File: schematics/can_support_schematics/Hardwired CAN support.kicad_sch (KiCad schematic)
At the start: 27 parts, among them J1 Programming Connector, J2 Conn_01x05_Male, J3 Conn_01x05_Male, J4 Screw_Terminal_01x02, J5 Screw_Terminal_01x04, SW1 SW_DIP_x04, U1 PIC18F26K83, U2 TCAN1042VDQ1, Y1 Crystal

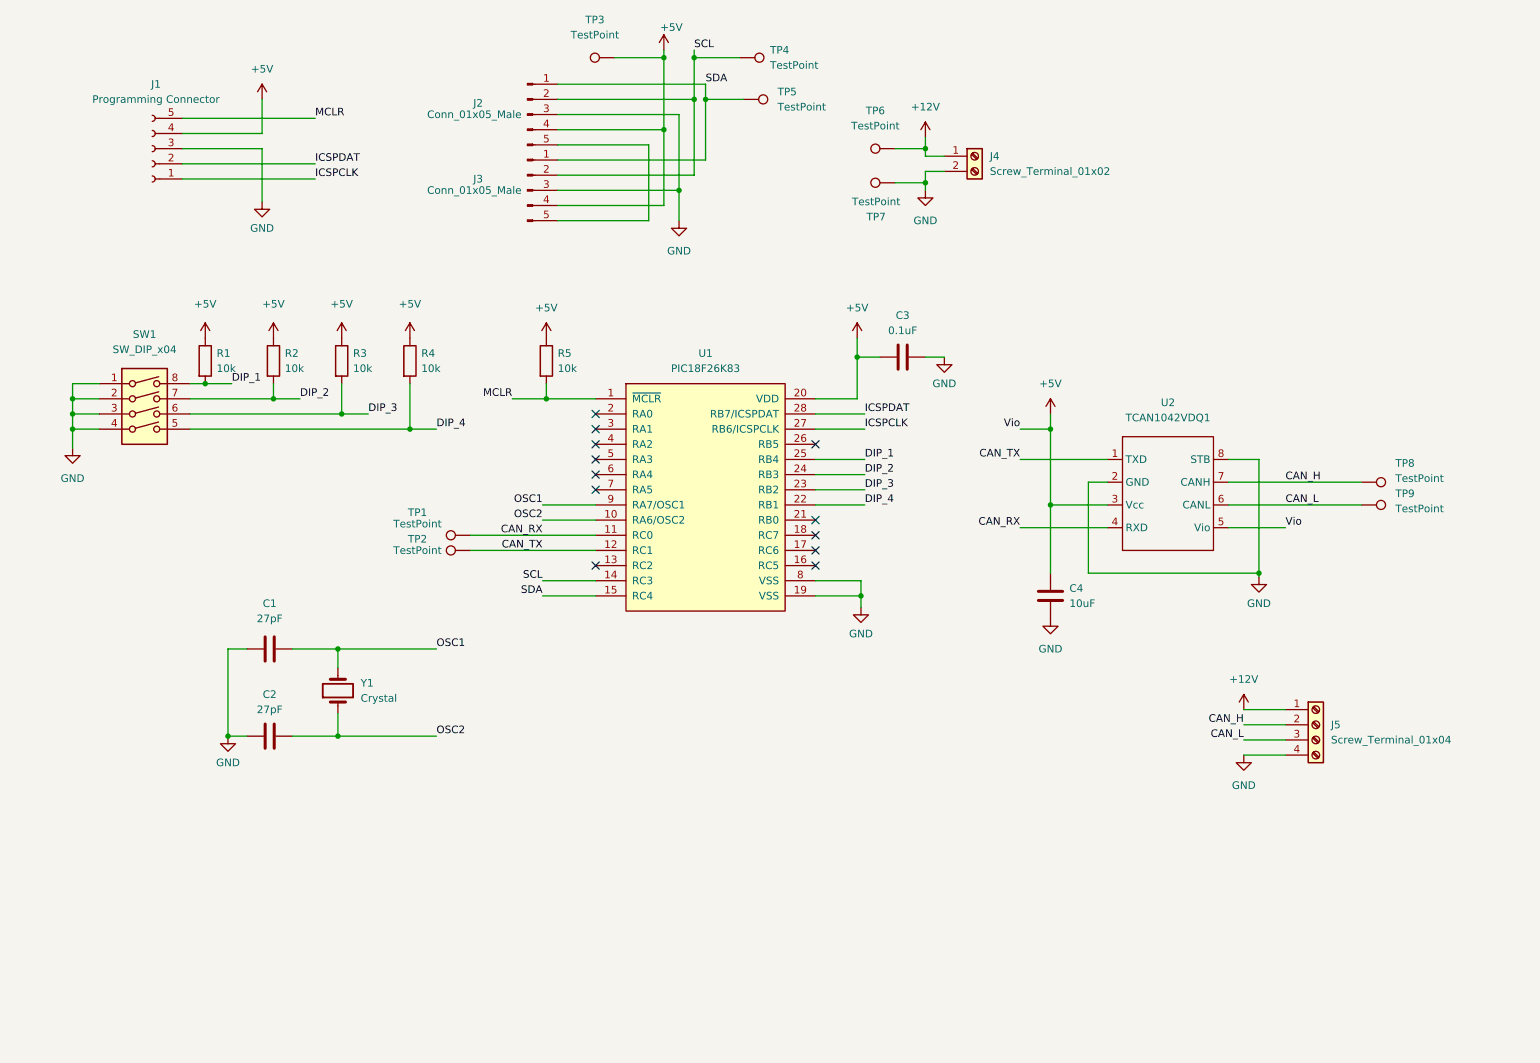
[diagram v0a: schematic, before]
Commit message: Stuff Updated
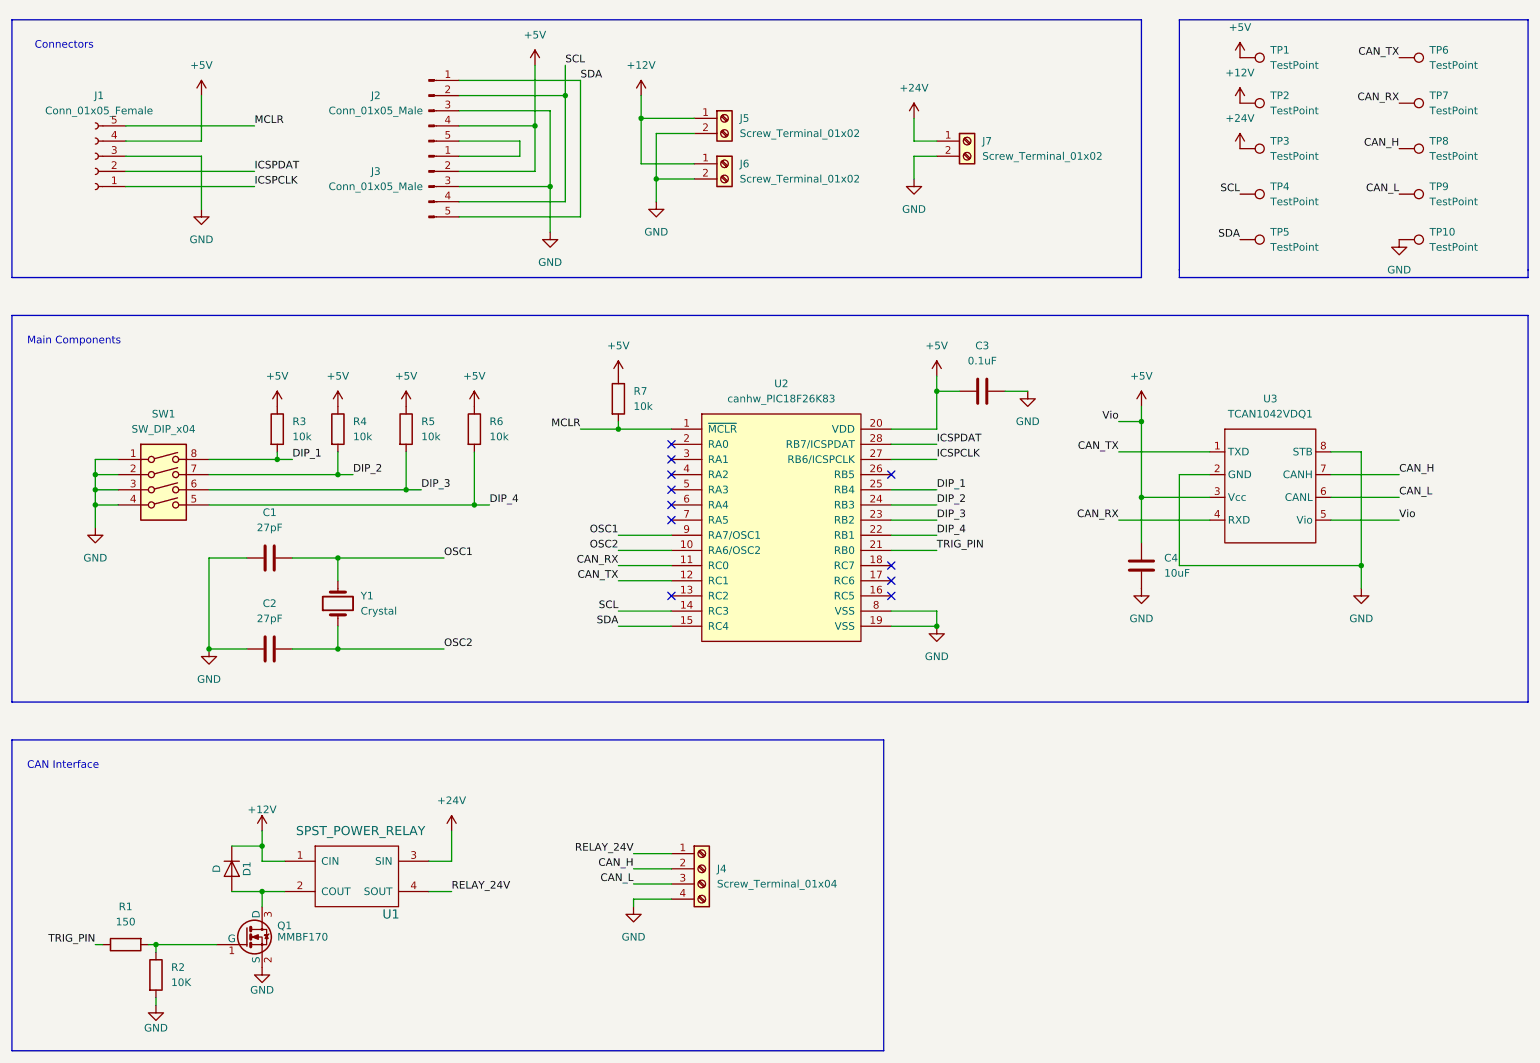
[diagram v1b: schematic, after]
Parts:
- removed J4: Screw_Terminal_01x02, symbol Connector:Screw_Terminal_01x02
- removed J5: Screw_Terminal_01x04, symbol Connector:Screw_Terminal_01x04
- removed U1: PIC18F26K83, symbol canhw:PIC18F26K83
- removed U2: TCAN1042VDQ1, symbol Hardwired CAN supp:TCAN1042VDQ1
- added D1: D, Diode_THT:D_DO-41_SOD81_P5.08mm_Vertical_AnodeUp, symbol rlcsv3_modular-rescue:D-rlcsv3_modular-rescue
- added J4: Screw_Terminal_01x04, TerminalBlock_Phoenix:TerminalBlock_Phoenix_MKDS-1,5-4-5.08_1x04_P5.08mm_Horizontal, symbol Connector:Screw_Terminal_01x04
- added J5, J6, J7: Screw_Terminal_01x02, TerminalBlock_Phoenix:TerminalBlock_Phoenix_MKDS-1,5-2-5.08_1x02_P5.08mm_Horizontal, symbol Connector:Screw_Terminal_01x02
- added Q1: MMBF170, Package_TO_SOT_SMD:SOT-23_Handsoldering, symbol rlcsv3_modular-rescue:MMBF170-rlcsv3_modular-rescue
- added R6, R7: 10k, Resistor_SMD:R_0805_2012Metric, symbol Device:R
- added TP10: TestPoint, TestPoint:TestPoint_THTPad_2.0x2.0mm_Drill1.0mm, symbol Connector:TestPoint
- added U1: SPST_POWER_RELAY, custom:Relay_SPST_G5LE-1A, symbol rlcsv3_modular-rescue:SPST_POWER_RELAY-rlcsv3_modular-rescue
- added U2: canhw_PIC18F26K83, Package_SO:SOIC-28W_7.5x17.9mm_P1.27mm, symbol actuator-cache[1]:canhw_PIC18F26K83
- added U3: TCAN1042VDQ1, Package_SO:SOIC-8_3.9x4.9mm_P1.27mm, symbol Hardwired CAN supp:TCAN1042VDQ1
- C1, C2, C3, C4: footprint (none) -> Capacitor_SMD:C_0805_2012Metric
- J1: value Programming Connector -> Conn_01x05_Female; footprint (none) -> canhw_footprints:PinHeader_5x2.54_SMD_90deg_952-3198-1-ND
- J2, J3: footprint (none) -> Connector_JST:JST_XH_S5B-XH-A-1_1x05_P2.50mm_Horizontal
- R1: value 10k -> 150; footprint (none) -> Resistor_SMD:R_0805_2012Metric
- R2: value 10k -> 10K; footprint (none) -> Resistor_SMD:R_0805_2012Metric
- R3, R4, R5: footprint (none) -> Resistor_SMD:R_0805_2012Metric
- SW1: footprint (none) -> custom:DIP_SWITCH_4X2
- TP1, TP2, TP3, TP4, TP5, TP6, TP7, TP8, TP9: footprint (none) -> TestPoint:TestPoint_THTPad_2.0x2.0mm_Drill1.0mm
- Y1: footprint (none) -> Crystal:Crystal_HC49-4H_Vertical
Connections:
- net +12V: now also TP2.1, D1.1 (K), J5.1 (Pin_1), J6.1 (Pin_1), U1.1 (CIN); no longer TP6.1
- net +5V: now also J3.2 (Pin_2), TP1.1, R6.1, R7.1, U2.20 (VDD), U3.3 (Vcc), U3.5 (Vio); no longer J3.4 (Pin_4), R1.1, R2.1, TP3.1
- net CAN_H: now also J4.2 (Pin_2), U3.7 (CANH)
- net CAN_L: now also J4.3 (Pin_3), U3.6 (CANL)
- net CAN_RX: now also TP7.1, U2.11 (RC0), U3.4 (RXD); no longer TP1.1
- net CAN_TX: now also TP6.1, U2.12 (RC1), U3.1 (TXD); no longer TP2.1
- net DIP_1: now also R3.2, U2.25 (RB4); no longer R1.2
- net DIP_2: now also R4.2, U2.24 (RB3); no longer R2.2
- net DIP_3: now also R5.2, U2.23 (RB2); no longer R3.2
- net DIP_4: now also R6.2, U2.22 (RB1); no longer R4.2
- net GND: now also C1.2, C2.2, R2.2, J4.4 (Pin_4), J5.2 (Pin_2), J6.2 (Pin_2), J7.2 (Pin_2), Q1.2 (S), TP10.1, U2.19 (VSS), U2.8 (VSS), U3.2 (GND), U3.8 (STB); no longer C1.1, C2.1, TP7.1
- net ICSPCLK: now also U2.27 (RB6/ICSPCLK)
- net ICSPDAT: now also U2.28 (RB7/ICSPDAT)
- net MCLR: now also R7.2, U2.1 (~{MCLR}); no longer R5.2
- net OSC1: now also C1.1, U2.9 (RA7/OSC1); no longer C1.2
- net OSC2: now also C2.1, U2.10 (RA6/OSC2); no longer C2.2
- net SCL: now also J3.4 (Pin_4), U2.14 (RC3); no longer J3.2 (Pin_2)
- net SDA: now also J3.5 (Pin_5), U2.15 (RC4); no longer J3.1 (Pin_1)
- net at J2.5 (Pin_5): now also J3.1 (Pin_1); no longer J3.5 (Pin_5)
- new net: Q1.1 (G), R1.2, R2.1
- new net: D1.2 (A), Q1.3 (D), U1.2 (COUT)
- new net +24V: J7.1 (Pin_1), TP3.1, U1.3 (SIN)
- new net RELAY_24V: J4.1 (Pin_1), U1.4 (SOUT)
- new net TRIG_PIN: R1.1, U2.21 (RB0)
- no-connect marks 12 -> 11
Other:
- note added: "CAN Interface"
- note added: "Connectors"
- note added: "Main Components"
